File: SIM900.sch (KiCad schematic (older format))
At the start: 72 parts, among them J1 Conn_01x05, J11 Conn_Coaxial_Power, J12 AudioJack2_Ground, J13 AudioJack2_Ground, J2 Conn_01x04, J3 Conn_01x04, J4 Conn_01x06, J5 Conn_01x02, J6 Conn_01x06, J7 Conn_01x03, J8 Conn_Coaxial_x2_Isolated, J9 SIM_Card, Q1 Q_NPN_BCE, Q2 Q_NPN_BCE, Q3 Q_NPN_BCE, SW1 SW_Push, U1 MIC29302WT, U2 SIM900

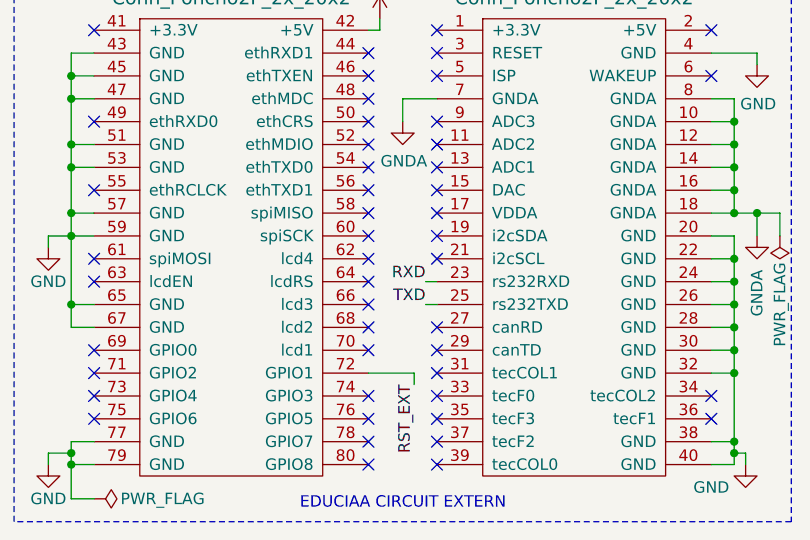
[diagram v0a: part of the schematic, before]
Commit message: Se realizaron los cambios a los comentarios hechos por el profesor
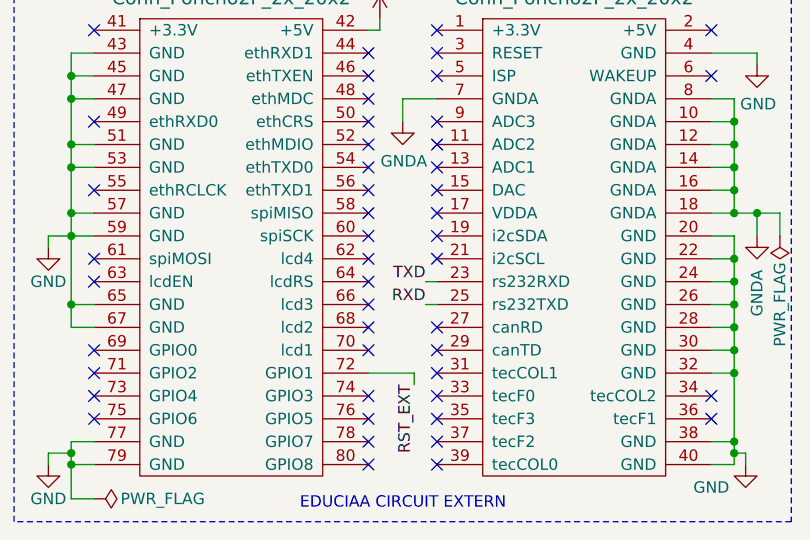
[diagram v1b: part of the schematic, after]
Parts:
- C1, C10, C11, C12, C13, C14, C15, C16, C17, C18, C19, C2, C20, C3, C4, C5, C6, C7, C8: Digikey (none) -> 399-17617-2-ND
- C9: Degikey (none) -> 399-17617-2-ND
- D1, D11, D2, D4: Digikey (none) -> SMAJ22CAQ-13-FDITR-ND
- D10, D8, D9: Digikey (none) -> BZD27C16P-E3-08GITR-ND
- D3: Digikey (none) -> 2460-L171L-QYC-TR-ND
- D5: Digokey (none) -> SMAJ22CAQ-13-FDITR-ND
- D6: Digikey (none) -> 2460-L171L-LICTR-ND
- D7: Field4 (none) -> BZD27C16P-E3-08GITR-ND
- J1: Digikey (none) -> S6103-ND
- J11: Digikey (none) -> H9161DKR-ND
- J12, J13: Digikey (none) -> CP-SJ2-35813B-SMT-DKR-ND
- J2, J3: Digikey (none) -> S9009E-04-ND
- J4, J6: Digikey (none) -> S7004-ND
- J7: Digikey (none) -> S9008E-03-ND
- J8: Digikey (none) -> 2057-RF2-49B-T-00-50-G-HDW-ND
- J9: Digikey (none) -> WM6698DKR-ND
- L1: footprint Inductor_SMD:L_0603_1608Metric_Pad1.05x0.95mm_HandSolder -> Inductor_SMD:L_0805_2012Metric; Digikey (none) -> 490-LQW2BAS6N0J00LDKR-ND
- Q1, Q2, Q3: Digikey (none) -> BC848BHZGT116DKR-ND
- R1, R10, R11, R12, R13, R15, R2, R3, R4, R5, R6, R7, R8: Digikey (none) -> 73L3R10JTR-ND
- R9: Degikey (none) -> 73L3R10JTR-ND
- U1: Digikey (none) -> 576-1124-ND
- U2: Digikey (none) -> 1597-1231-ND
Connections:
- net RXD: now also XA1.25 (rs232TXD); no longer XA1.23 (rs232RXD)
- net TXD: now also XA1.23 (rs232RXD); no longer XA1.25 (rs232TXD)
